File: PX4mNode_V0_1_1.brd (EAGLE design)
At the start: 48.6 x 34.9 mm, 135 parts, among them J201 DF13C-6P-1.25V, J202 DF13C-6P-1.25V, J203 DF13C-6P-1.25V, J301 DF13C-4P-1.25V, J401 DF13C-7P-1.25V, J402 DF13-4P-1.25V, J403 DF13C-4P-1.25V, J404 DF13C-4P-1.25V, J405 DF13C-4P-1.25V, J801 DF13C-3P-1.25V, M3_MOUNT1101 MOUNT-HOLE3.1MM, M3_MOUNT1102 MOUNT-HOLE3.1MM, M3_MOUNT1103 MOUNT-HOLE3.1MM, M3_MOUNT1104 MOUNT-HOLE3.1MM, U101 STM32F4X7VX, U401 MAX3051, U402 MAX3051, X101 3.2x2.5 mm / 24 MHz / 15 ppm

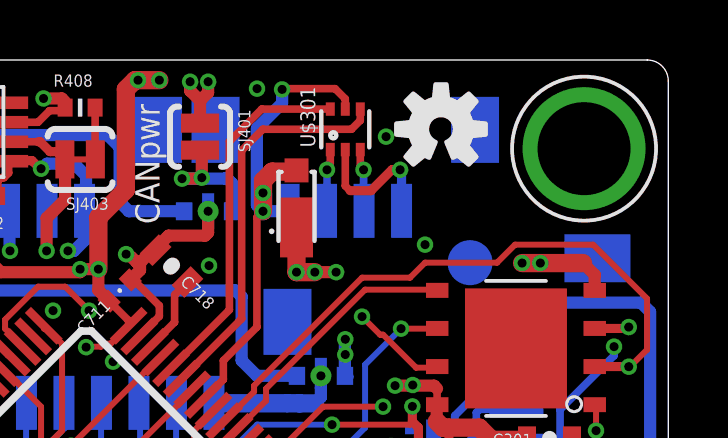
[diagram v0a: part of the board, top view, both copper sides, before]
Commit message: Graphic shuffle
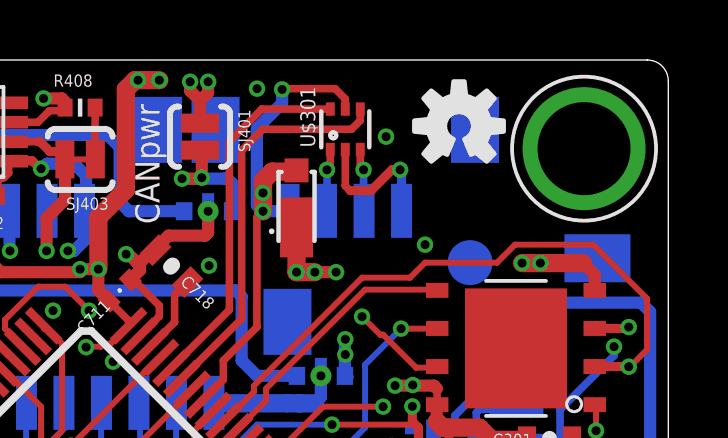
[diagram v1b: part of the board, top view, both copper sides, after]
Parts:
- moved OSHW_LOGO 0.61 mm to (50.8, 35.5)
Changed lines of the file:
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@@
 <layer number="17" name="Pads" color="2" fill="1" visible="yes" active="yes"/>
 <layer number="18" name="Vias" color="2" fill="1" visible="yes" active="yes"/>
-<layer number="19" name="Unrouted" color="14" fill="1" visible="no" active="yes"/>
+<layer number="19" name="Unrouted" color="14" fill="1" visible="yes" active="yes"/>
 <layer number="20" name="Dimension" color="15" fill="1" visible="yes" active="yes"/>
 <layer number="21" name="tPlace" color="7" fill="1" visible="no" active="yes"/>
@@
 <attribute name="PARTNO" value="DF13C-6P-1.25V(20)" x="38.716" y="6.864" size="1.778" layer="28" rot="MR0" display="off"/>
 </element>
-<element name="OSHW_LOGO" library="pixhawk2" package="OSHW-LOGO-S" value="OSHW-LOGOS" x="50.2312" y="35.352">
-<attribute name="PARTNO" value="*" x="50.2312" y="46.528" size="1.778" layer="27" display="off"/>
-<attribute name="BOM" value="EXCLUDE" x="50.2312" y="46.528" size="1.778" layer="27" display="off"/>
+<element name="OSHW_LOGO" library="pixhawk2" package="OSHW-LOGO-S" value="OSHW-LOGOS" x="50.8312" y="35.452">
+<attribute name="PARTNO" value="*" x="50.8312" y="46.628" size="1.778" layer="27" display="off"/>
+<attribute name="BOM" value="EXCLUDE" x="50.8312" y="46.628" size="1.778" layer="27" display="off"/>
 </element>
 <element name="M3_MOUNT1104" library="pixhawk2" package="MOUNT-HOLE3.1" value="MOUNT-HOLE3.1MM" x="12.2" y="5.7" locked="yes">
